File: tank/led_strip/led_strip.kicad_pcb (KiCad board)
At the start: 2 copper layers, 55 x 10.8 mm, 9 parts, among them J1 Conn_01x04_Male

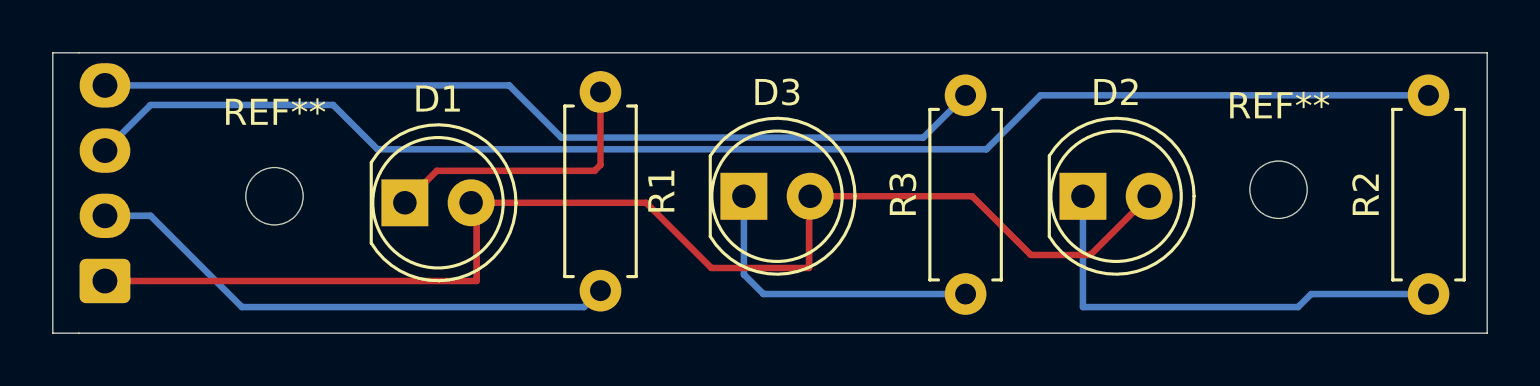
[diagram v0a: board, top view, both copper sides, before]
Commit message: and all that jazz
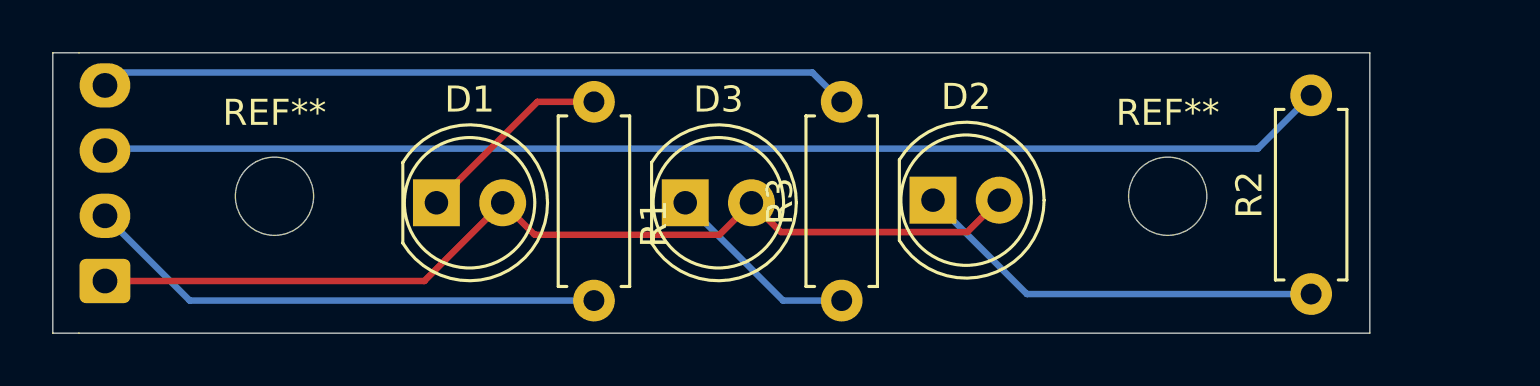
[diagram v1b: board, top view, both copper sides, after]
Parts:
- moved D2 5.75 mm to (126.8, 97.9)
- moved R3 4.76 mm to (123.2, 101.8)
- moved R2 4.50 mm to (141.2, 101.5)
- moved REF** 4.26 mm to (135.8, 97.8)
- moved D3 2.26 mm to (117.2, 98.0)
- moved D1 1.21 mm to (107.7, 98.0)
- moved R1 0.45 mm to (113.8, 94.1)
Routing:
- net Net-(D1-Pad2): track 49.0 -> 37.5 mm
- net Net-(J1-Pad3): track 53.0 -> 47.1 mm
- net Net-(J1-Pad4): track 34.5 -> 28.9 mm
- net Net-(D3-Pad1): track 11.8 -> 7.55 mm
- net Net-(D1-Pad1): track 10.9 -> 7.64 mm
- net Net-(D2-Pad1): track 17.7 -> 16.0 mm
- net Net-(J1-Pad2): track 20.7 -> 20.1 mm
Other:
- board size 55 x 10.8 mm -> 50.5 x 10.8 mm
- board text added: "LED Strip Version 0.4"
- board text removed: "LED Strip Version 0.3"
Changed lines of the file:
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@@
     (thickness 1.6)
     (drawings 8)
-    (tracks 37)
+    (tracks 22)
     (zones 0)
     (modules 9)
@@
     (mod_text_size 1 1)
     (mod_text_width 0.15)
-    (pad_size 1.524 1.524)
-    (pad_drill 0.762)
+    (pad_size 3 3)
+    (pad_drill 3)
     (pad_to_mask_clearance 0.05)
     (aux_axis_origin 0 0)
@@
       (effects (font (size 1 1) (thickness 0.15)))
     )
-    (pad 1 np_thru_hole circle (at 0 0) (size 2.2 2.2) (drill 2.2) (layers *.Cu *.Mask))
+    (pad "" np_thru_hole circle (at 0 0) (size 3 3) (drill 3) (layers *.Cu *.Mask))
   )
   (module MountingHole:MountingHole_2.2mm_M2 (layer F.Cu)
-    (at 140 97.5)
+    (at 135.75 97.75)
     (descr "Mounting Hole 2.2mm, no annular, M2")
     (tags "mounting hole 2.2mm no annular m2")
@@
       (effects (font (size 1 1) (thickness 0.15)))
     )
-    (pad 1 np_thru_hole circle (at 0 0) (size 2.2 2.2) (drill 2.2) (layers *.Cu *.Mask))
+    (pad "" np_thru_hole circle (at 0 0) (size 3 3) (drill 3) (layers *.Cu *.Mask))
   )
   (module LED_THT:LED_D5.0mm (layer F.Cu)
-    (at 106.5 98)
+    (at 107.71 98)
     (descr "LED, diameter 5.0mm, 2 pins, http://cdn-reichelt.de/documents/datenblatt/A500/LL-504BC2E-009.pdf")
     (tags "LED diameter 5.0mm 2 pins")
@@
   )
   (module LED_THT:LED_D5.0mm (layer F.Cu)
-    (at 132.5 97.75)
+    (at 126.75 97.9)
     (descr "LED, diameter 5.0mm, 2 pins, http://cdn-reichelt.de/documents/datenblatt/A500/LL-504BC2E-009.pdf")
     (tags "LED diameter 5.0mm 2 pins")
@@
   )
   (module LED_THT:LED_D5.0mm (layer F.Cu)
-    (at 119.5 97.75)
+    (at 117.25 98)
     (descr "LED, diameter 5.0mm, 2 pins, http://cdn-reichelt.de/documents/datenblatt/A500/LL-504BC2E-009.pdf")
     (tags "LED diameter 5.0mm 2 pins")
@@
   )
   (module Resistor_THT:R_Axial_DIN0207_L6.3mm_D2.5mm_P7.62mm_Horizontal (layer F.Cu)
-    (at 114 93.75 270)
+    (at 113.75 94.13 270)
     (descr "Resistor, Axial_DIN0207 series, Axial, Horizontal, pin pitch=7.62mm, 0.25W = 1/4W, length*diameter=6.3*2.5mm^2, http://cdn-reichelt.de/documents/datenblatt/B400/1_4W%23YAG.pdf")
     (tags "Resistor Axial_DIN0207 series Axial Horizontal pin pitch 7.62mm 0.25W = 1/4W length 6.3mm diameter 2.5mm")
-    (fp_text reference R1 (at 3.81 -2.37 90) (layer F.SilkS)
+    (fp_text reference R1 (at 4.67 -2.3 90) (layer F.SilkS)
       (effects (font (size 1 1) (thickness 0.15)))
     )
@@
   )
   (module Resistor_THT:R_Axial_DIN0207_L6.3mm_D2.5mm_P7.62mm_Horizontal (layer F.Cu)
-    (at 145.75 101.5 90)
+    (at 141.25 101.5 90)
     (descr "Resistor, Axial_DIN0207 series, Axial, Horizontal, pin pitch=7.62mm, 0.25W = 1/4W, length*diameter=6.3*2.5mm^2, http://cdn-reichelt.de/documents/datenblatt/B400/1_4W%23YAG.pdf")
     (tags "Resistor Axial_DIN0207 series Axial Horizontal pin pitch 7.62mm 0.25W = 1/4W length 6.3mm diameter 2.5mm")
@@
   )
   (module Resistor_THT:R_Axial_DIN0207_L6.3mm_D2.5mm_P7.62mm_Horizontal (layer F.Cu)
-    (at 128 101.5 90)
+    (at 123.25 101.75 90)
     (descr "Resistor, Axial_DIN0207 series, Axial, Horizontal, pin pitch=7.62mm, 0.25W = 1/4W, length*diameter=6.3*2.5mm^2, http://cdn-reichelt.de/documents/datenblatt/B400/1_4W%23YAG.pdf")
     (tags "Resistor Axial_DIN0207 series Axial Horizontal pin pitch 7.62mm 0.25W = 1/4W length 6.3mm diameter 2.5mm")
@@
     (effects (font (size 1 1) (thickness 0.15)) (justify mirror))
   )
-  (gr_text "LED Strip Version 0.3" (at 120.75 99.5) (layer B.SilkS)
+  (gr_text "LED Strip Version 0.4" (at 120.75 99.5) (layer B.SilkS)
     (effects (font (size 1 1) (thickness 0.15)) (justify mirror))
   )
   (gr_line (start 93 103) (end 93 92.25) (layer Edge.Cuts) (width 0.05))
-  (gr_line (start 148 103) (end 94 103) (layer Edge.Cuts) (width 0.05))
-  (gr_line (start 148 92.25) (end 148 103) (layer Edge.Cuts) (width 0.05))
-  (gr_line (start 94 92.25) (end 148 92.25) (layer Edge.Cuts) (width 0.05))
-  (segment (start 107.725001 96.774999) (end 113.774999 96.774999) (width 0.25) (layer F.Cu) (net 1))
-  (segment (start 106.5 98) (end 107.725001 96.774999) (width 0.25) (layer F.Cu) (net 1))
-  (segment (start 114 96.549998) (end 114 93.75) (width 0.25) (layer F.Cu) (net 1))
-  (segment (start 113.774999 96.774999) (end 114 96.549998) (width 0.25) (layer F.Cu) (net 1))
-  (segment (start 95 101) (end 109.25 101) (width 0.25) (layer F.Cu) (net 2))
-  (segment (start 109.25 98.21) (end 109.04 98) (width 0.25) (layer F.Cu) (net 2))
-  (segment (start 109.25 101) (end 109.25 98.21) (width 0.25) (layer F.Cu) (net 2))
-  (segment (start 109.04 98) (end 115.75 98) (width 0.25) (layer F.Cu) (net 2))
-  (segment (start 115.75 98) (end 118.25 100.5) (width 0.25) (layer F.Cu) (net 2))
-  (segment (start 118.25 100.5) (end 122 100.5) (width 0.25) (layer F.Cu) (net 2))
-  (segment (start 122 97.79) (end 122.04 97.75) (width 0.25) (layer F.Cu) (net 2))
-  (segment (start 122 100.5) (end 122 97.79) (width 0.25) (layer F.Cu) (net 2))
-  (segment (start 122.04 97.75) (end 128.25 97.75) (width 0.25) (layer F.Cu) (net 2))
-  (segment (start 128.25 97.75) (end 130.5 100) (width 0.25) (layer F.Cu) (net 2))
-  (segment (start 132.79 100) (end 135.04 97.75) (width 0.25) (layer F.Cu) (net 2))
-  (segment (start 130.5 100) (end 132.79 100) (width 0.25) (layer F.Cu) (net 2))
-  (segment (start 95 98.5) (end 96.75 98.5) (width 0.25) (layer B.Cu) (net 3))
-  (segment (start 96.75 98.5) (end 100.25 102) (width 0.25) (layer B.Cu) (net 3))
-  (segment (start 113.37 102) (end 114 101.37) (width 0.25) (layer B.Cu) (net 3))
-  (segment (start 100.25 102) (end 113.37 102) (width 0.25) (layer B.Cu) (net 3))
-  (segment (start 103.75 94.25) (end 96.75 94.25) (width 0.25) (layer B.Cu) (net 4))
-  (segment (start 105.45001 95.95001) (end 103.75 94.25) (width 0.25) (layer B.Cu) (net 4))
-  (segment (start 128.79999 95.95001) (end 105.45001 95.95001) (width 0.25) (layer B.Cu) (net 4))
-  (segment (start 96.75 94.25) (end 95 96) (width 0.25) (layer B.Cu) (net 4))
-  (segment (start 130.87 93.88) (end 128.79999 95.95001) (width 0.25) (layer B.Cu) (net 4))
-  (segment (start 145.75 93.88) (end 130.87 93.88) (width 0.25) (layer B.Cu) (net 4))
-  (segment (start 95 93.5) (end 110.5 93.5) (width 0.25) (layer B.Cu) (net 5))
-  (segment (start 110.5 93.5) (end 112.5 95.5) (width 0.25) (layer B.Cu) (net 5))
-  (segment (start 126.38 95.5) (end 128 93.88) (width 0.25) (layer B.Cu) (net 5))
-  (segment (start 112.5 95.5) (end 126.38 95.5) (width 0.25) (layer B.Cu) (net 5))
-  (segment (start 132.5 97.75) (end 132.5 102) (width 0.25) (layer B.Cu) (net 6))
-  (segment (start 141.25 101.5) (end 145.75 101.5) (width 0.25) (layer B.Cu) (net 6))
-  (segment (start 140.75 102) (end 141.25 101.5) (width 0.25) (layer B.Cu) (net 6))
-  (segment (start 132.5 102) (end 140.75 102) (width 0.25) (layer B.Cu) (net 6))
-  (segment (start 119.5 97.75) (end 119.5 100.75) (width 0.25) (layer B.Cu) (net 7))
-  (segment (start 120.25 101.5) (end 128 101.5) (width 0.25) (layer B.Cu) (net 7))
-  (segment (start 119.5 100.75) (end 120.25 101.5) (width 0.25) (layer B.Cu) (net 7))
+  (gr_line (start 143.5 103) (end 94 103) (layer Edge.Cuts) (width 0.05))
+  (gr_line (start 143.5 92.25) (end 143.5 103) (layer Edge.Cuts) (width 0.05))
+  (gr_line (start 94 92.25) (end 143.5 92.25) (layer Edge.Cuts) (width 0.05))
+  (segment (start 111.58 94.13) (end 113.75 94.13) (width 0.25) (layer F.Cu) (net 1))
+  (segment (start 107.71 98) (end 111.58 94.13) (width 0.25) (layer F.Cu) (net 1))
+  (segment (start 107.25 101) (end 110.25 98) (width 0.25) (layer F.Cu) (net 2))
+  (segment (start 95 101) (end 107.25 101) (width 0.25) (layer F.Cu) (net 2))
+  (segment (start 118.564999 99.225001) (end 119.79 98) (width 0.25) (layer F.Cu) (net 2))
+  (segment (start 111.475001 99.225001) (end 118.564999 99.225001) (width 0.25) (layer F.Cu) (net 2))
+  (segment (start 110.25 98) (end 111.475001 99.225001) (width 0.25) (layer F.Cu) (net 2))
+  (segment (start 128.064999 99.125001) (end 129.29 97.9) (width 0.25) (layer F.Cu) (net 2))
+  (segment (start 120.915001 99.125001) (end 128.064999 99.125001) (width 0.25) (layer F.Cu) (net 2))
+  (segment (start 119.79 98) (end 120.915001 99.125001) (width 0.25) (layer F.Cu) (net 2))
+  (segment (start 98.25 101.75) (end 113.75 101.75) (width 0.25) (layer B.Cu) (net 3))
+  (segment (start 95 98.5) (end 98.25 101.75) (width 0.25) (layer B.Cu) (net 3))
+  (segment (start 139.205001 95.924999) (end 141.25 93.88) (width 0.25) (layer B.Cu) (net 4))
+  (segment (start 95.075001 95.924999) (end 139.205001 95.924999) (width 0.25) (layer B.Cu) (net 4))
+  (segment (start 95 96) (end 95.075001 95.924999) (width 0.25) (layer B.Cu) (net 4))
+  (segment (start 122.124999 93.004999) (end 123.25 94.13) (width 0.25) (layer B.Cu) (net 5))
+  (segment (start 95.495001 93.004999) (end 122.124999 93.004999) (width 0.25) (layer B.Cu) (net 5))
+  (segment (start 95 93.5) (end 95.495001 93.004999) (width 0.25) (layer B.Cu) (net 5))
+  (segment (start 130.35 101.5) (end 141.25 101.5) (width 0.25) (layer B.Cu) (net 6))
+  (segment (start 126.75 97.9) (end 130.35 101.5) (width 0.25) (layer B.Cu) (net 6))
+  (segment (start 121 101.75) (end 123.25 101.75) (width 0.25) (layer B.Cu) (net 7))
+  (segment (start 117.25 98) (end 121 101.75) (width 0.25) (layer B.Cu) (net 7))
 )
